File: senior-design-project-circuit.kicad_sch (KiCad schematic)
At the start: 49 parts, among them J1 Micro_SD_Card, J10 Conn_01x01_Male, J11 Conn_01x01_Male, J12 Conn_01x01_Male, J15 Conn_01x01_Male, J2A1 Conn_01x15_Female, J2B1 Conn_01x15_Female, J3 Conn_01x16_Male, J4 USB_B_Micro, J5 Conn_01x02, J6 Conn_01x06_Female, J7 Conn_01x01_Male, J8 Conn_01x01_Male, J9 Conn_01x01_Male, SW1 SW_Push, SW2 SW_Push, SW3 SW_Push, U1 4050, U2 LM2594M-3.3, U3 MCP73831-2-OT

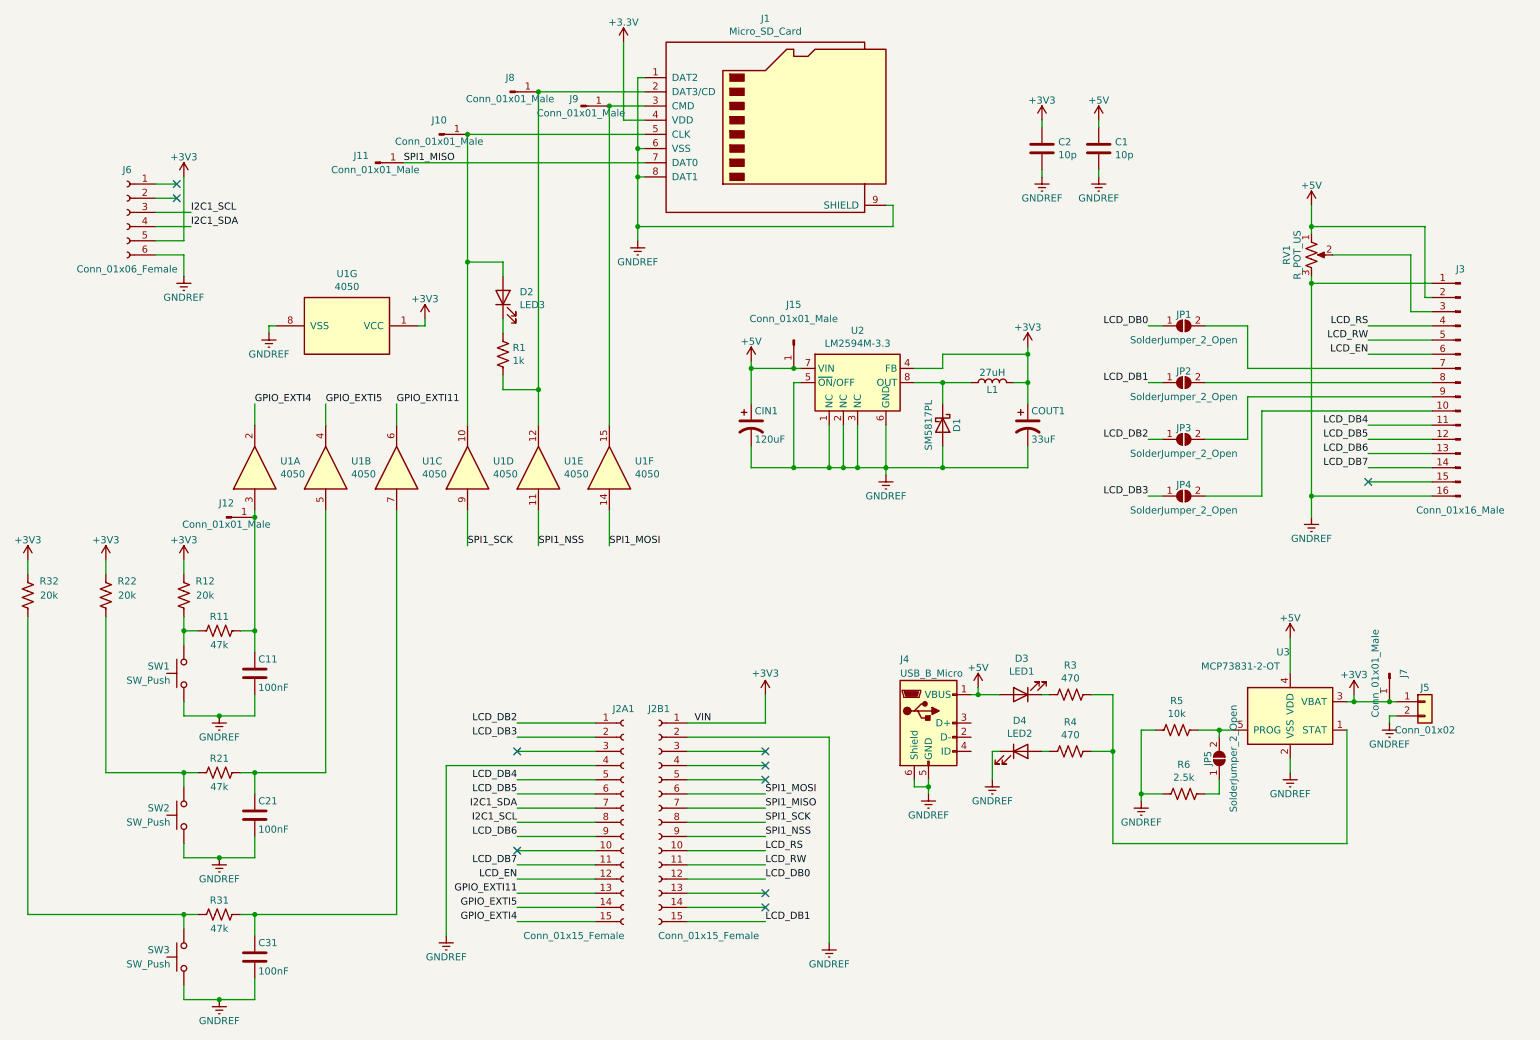
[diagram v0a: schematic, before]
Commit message: Add files via upload
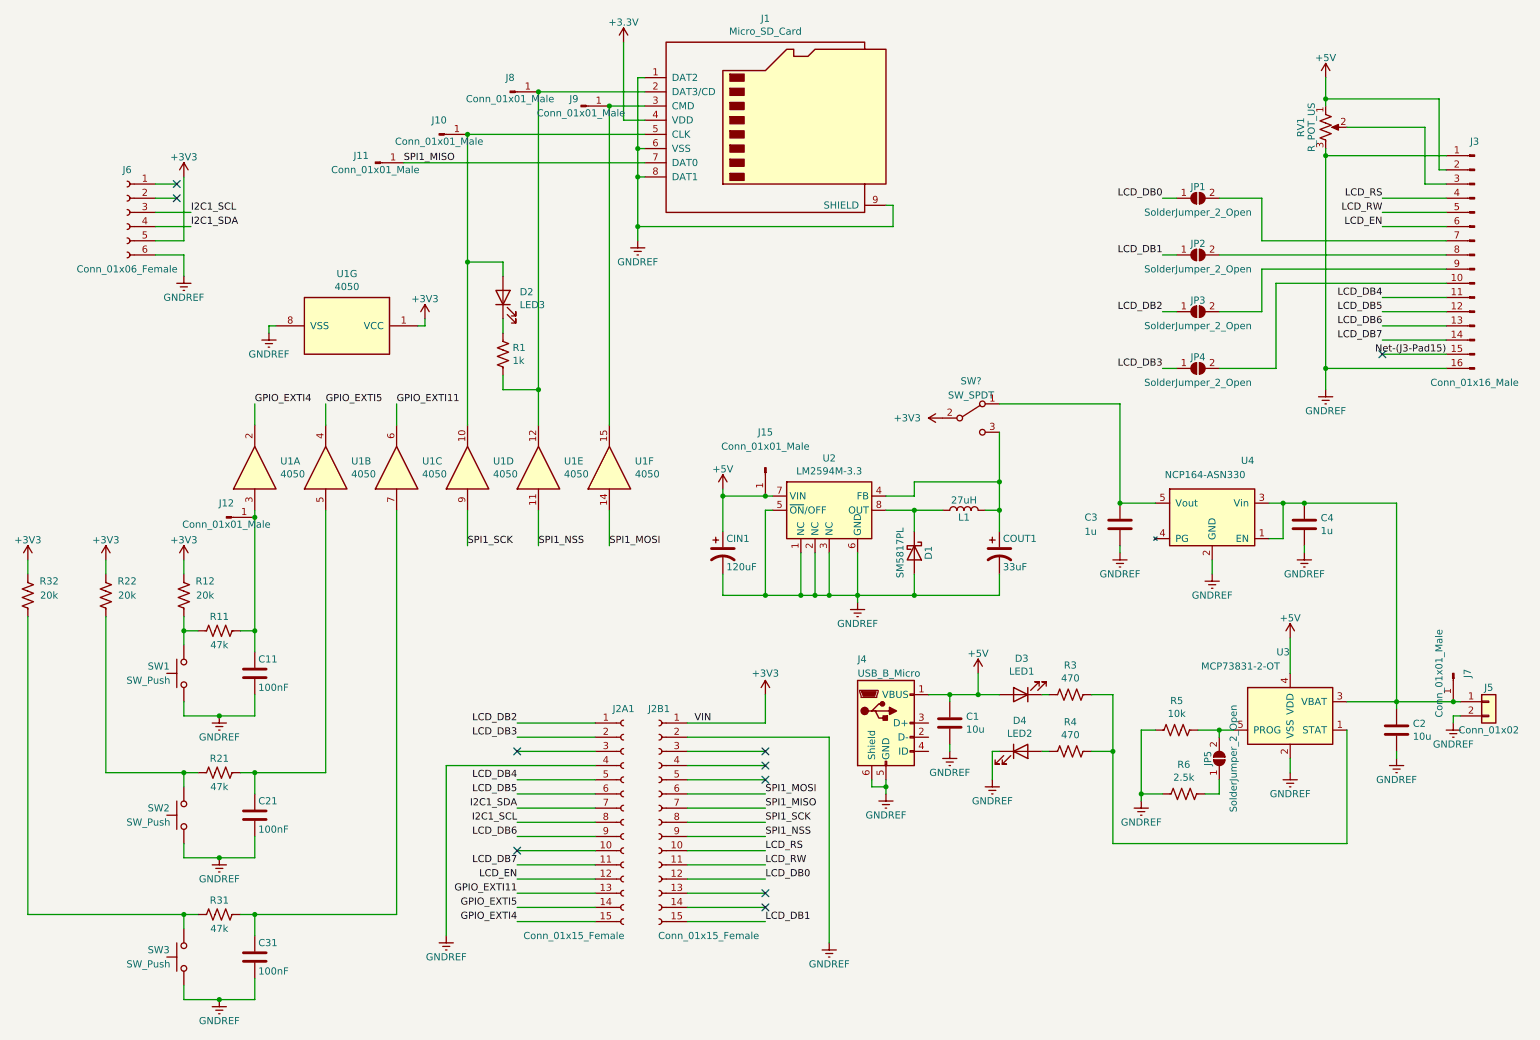
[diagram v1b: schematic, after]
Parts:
- added C3, C4: 1u, Capacitor_SMD:C_0603_1608Metric_Pad1.08x0.95mm_HandSolder, symbol Device:C
- added SW?: SW_SPDT, symbol Switch:SW_SPDT
- added U4: NCP164-ASN330, Package_TO_SOT_SMD:SOT-23-5, symbol Battery_Management:MCP73831-2-OT
- C1, C2: value 10p -> 10u
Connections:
- net +3V3: now also SW?.2 (B); no longer C2.1, COUT1.1, J5.1 (Pin_1), J7.1 (Pin_1), L1.2, U2.4 (FB), U3.3 (VBAT)
- net GNDREF: now also C3.2, C4.2, U4.2 (GND)
- net Net-(J3-Pad15): now reaches J3.15 (Pin_15)
- new net: COUT1.1, L1.2, SW?.3 (C), U2.4 (FB)
- new net: C2.1, C4.1, J5.1 (Pin_1), J7.1 (Pin_1), U3.3 (VBAT), U4.1 (EN), U4.3 (Vin)
- new net: C3.1, SW?.1 (A), U4.5 (Vout)
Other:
- moved on the sheet: C1, C2, CIN1, COUT1, D1, J15, J3, J4, J5, J7, JP1, JP2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
